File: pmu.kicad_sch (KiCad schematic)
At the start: 21 parts, among them J4 Battery, Q4 BSS138, Q5 BSS84, SW1 POWER ON, U3 MAX1555, U4 TPS63030DSK

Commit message: more pcb routing
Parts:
- C12, C13: footprint Capacitor_SMD:C_0805_2012Metric -> Capacitor_SMD:C_0402_1005Metric
- R11, R12, R13, R14, R15, R16: footprint Resistor_SMD:R_0805_2012Metric -> Resistor_SMD:R_0402_1005Metric
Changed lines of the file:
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@@
 			)
 		)
-		(property "Footprint" "Resistor_SMD:R_0805_2012Metric"
+		(property "Footprint" "Resistor_SMD:R_0402_1005Metric"
 			(at 119.888 115.57 90)
 			(effects
@@
 			)
 		)
-		(property "Footprint" "Resistor_SMD:R_0805_2012Metric"
+		(property "Footprint" "Resistor_SMD:R_0402_1005Metric"
 			(at 85.852 115.57 90)
 			(effects
@@
 			)
 		)
-		(property "Footprint" "Resistor_SMD:R_0805_2012Metric"
+		(property "Footprint" "Resistor_SMD:R_0402_1005Metric"
 			(at 141.478 113.03 90)
 			(effects
@@
 			)
 		)
-		(property "Footprint" "Capacitor_SMD:C_0805_2012Metric"
+		(property "Footprint" "Capacitor_SMD:C_0402_1005Metric"
 			(at 143.8148 95.25 0)
 			(effects
@@
 			)
 		)
-		(property "Footprint" "Resistor_SMD:R_0805_2012Metric"
+		(property "Footprint" "Resistor_SMD:R_0402_1005Metric"
 			(at 110.998 90.17 90)
 			(effects
@@
 			)
 		)
-		(property "Footprint" "Capacitor_SMD:C_0805_2012Metric"
+		(property "Footprint" "Capacitor_SMD:C_0402_1005Metric"
 			(at 91.7448 111.76 0)
 			(effects
@@
 			)
 		)
-		(property "Footprint" "Resistor_SMD:R_0805_2012Metric"
+		(property "Footprint" "Resistor_SMD:R_0402_1005Metric"
 			(at 81.28 107.442 90)
 			(effects
@@
 			)
 		)
-		(property "Footprint" "Resistor_SMD:R_0805_2012Metric"
+		(property "Footprint" "Resistor_SMD:R_0402_1005Metric"
 			(at 220.98 82.042 90)
 			(effects

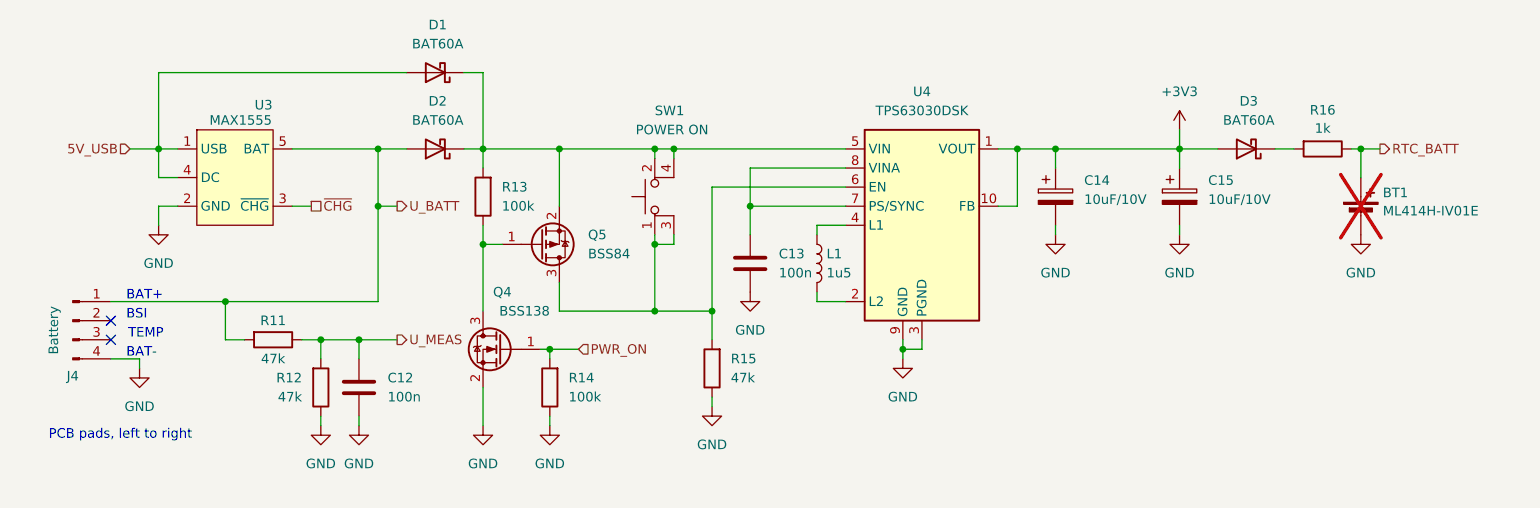
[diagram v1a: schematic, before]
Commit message: more pcb routing
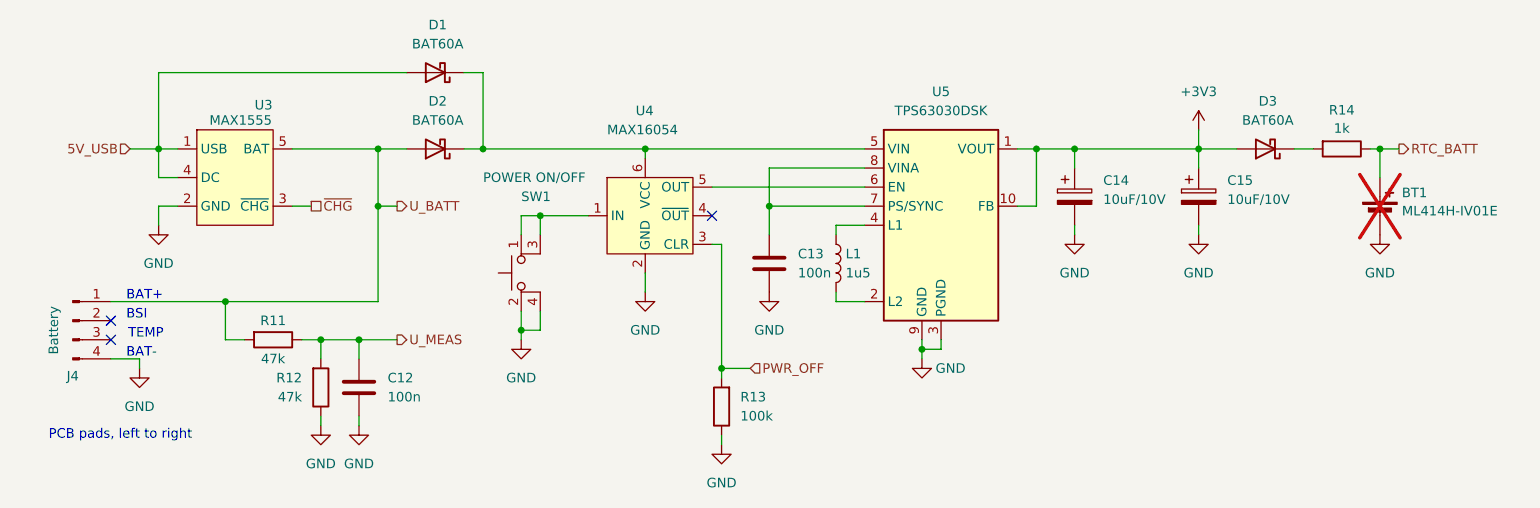
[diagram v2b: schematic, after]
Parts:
- removed Q4: BSS138, Package_TO_SOT_SMD:SOT-23, symbol Transistor_FET:BSS138
- removed Q5: BSS84, Package_TO_SOT_SMD:SOT-23, symbol Transistor_FET:BSS84
- removed R13: 100k, Resistor_SMD:R_0402_1005Metric, symbol Device:R
- removed R15: 47k, Resistor_SMD:R_0402_1005Metric, symbol Device:R
- added U4: MAX16054, Package_TO_SOT_SMD:TSOT-23-6, symbol Parts:MAX16054
- SW1: value POWER ON -> POWER ON/OFF
- renumbered R14 to R13, R16 to R14, U4 to U5
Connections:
- net GND: now also SW1.2, SW1.4 (A), U4.2 (GND)
- net at D1.1 (K), D2.1 (K), U5.5 (VIN): now also U4.6 (VCC); no longer SW1.2, SW1.4 (A)
- net at SW1.1, SW1.3 (K): now also U4.1 (IN); no longer U5.6 (EN)
- net PWR_ON renamed PWR_OFF
- net PWR_OFF: now also U4.3 (CLR)
- new net: U4.5 (OUT), U5.6 (EN)
- no-connect marks 2 -> 3
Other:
- moved on the sheet: BT1, C13, C14, C15, D3, L1, R13, R14, SW1, U5
